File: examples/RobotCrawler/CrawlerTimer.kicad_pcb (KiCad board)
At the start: 2 copper layers, 50 x 62 mm, 38 parts

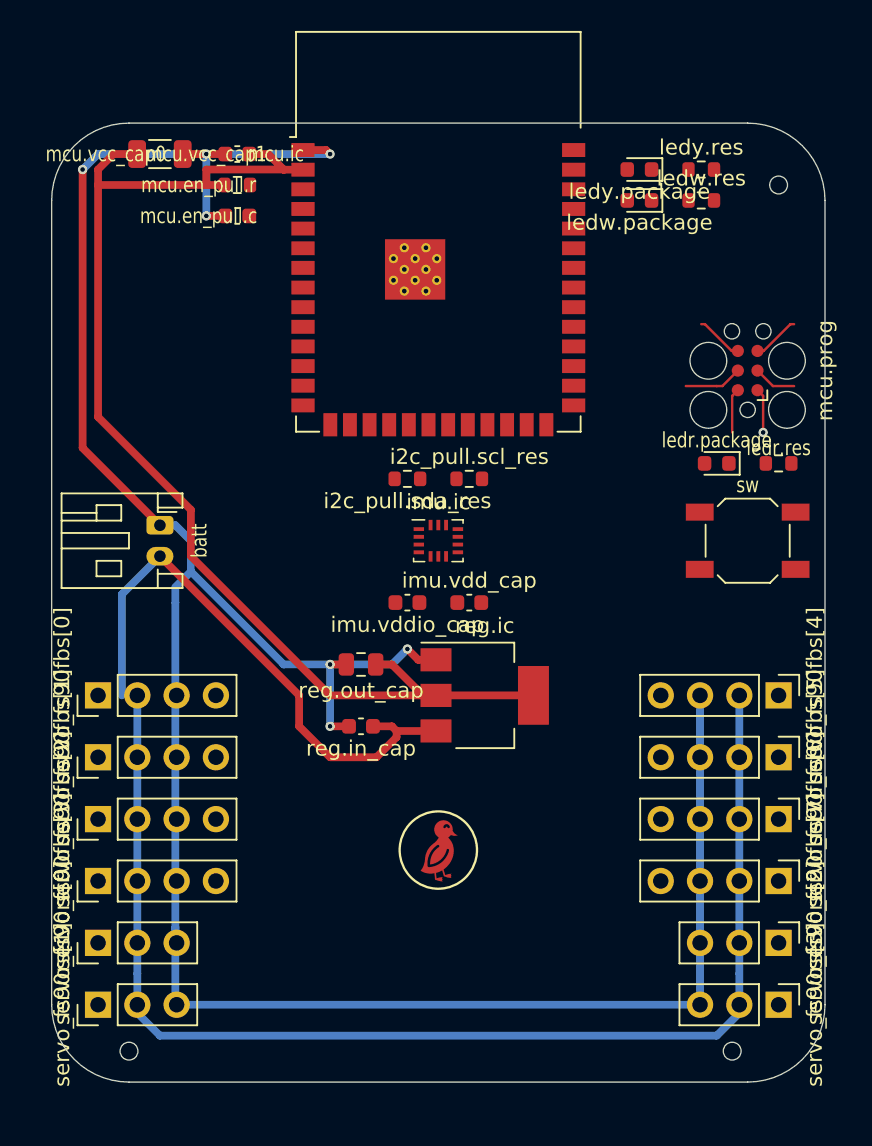
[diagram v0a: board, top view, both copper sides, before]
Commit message: just one copper duck given
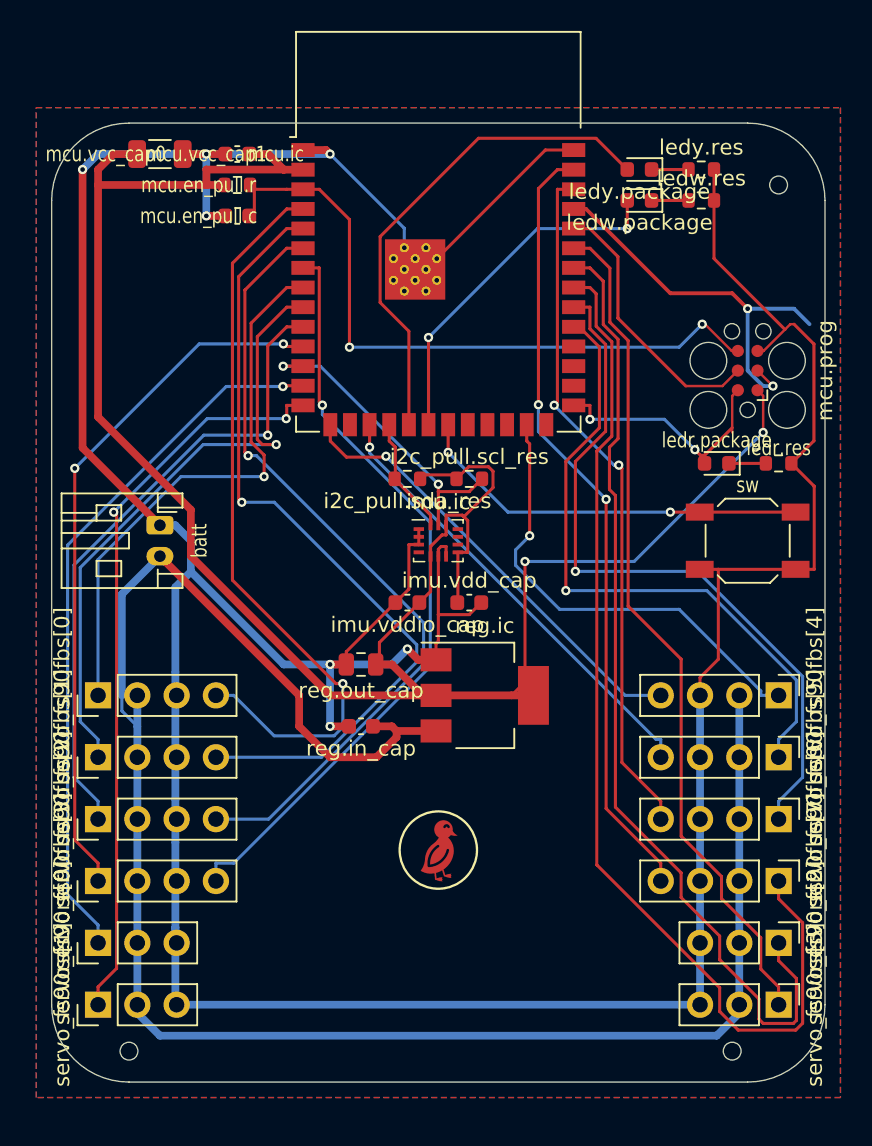
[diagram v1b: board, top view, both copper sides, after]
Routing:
- net batt.gnd: track 167.4 -> 277.2 mm
- net servo_fs90fbs[7].pwm: track 0.00 -> 68.0 mm
- net servo_fs90rs[2].pwm: track 0.00 -> 62.7 mm
- net imu.pwr: track 82.0 -> 138.0 mm, vias 1 -> 2
- net servo_fs90rs[3].pwm: track 0.00 -> 55.0 mm
- net servo_fs90fbs[1].fb: track 0.00 -> 51.9 mm, vias 0 -> 1
- net servo_fs90fbs[2].fb: track 0.00 -> 51.7 mm, vias 0 -> 1
- net servo_fs90fbs[7].fb: track 0.00 -> 50.8 mm, vias 0 -> 2
- net servo_fs90fbs[3].fb: track 0.00 -> 50.1 mm, vias 0 -> 1
- net servo_fs90fbs[0].fb: track 0.00 -> 48.7 mm, vias 0 -> 1
- net servo_fs90rs[1].pwm: track 0.00 -> 48.0 mm, vias 0 -> 2
- net servo_fs90fbs[6].pwm: track 0.00 -> 46.7 mm, vias 0 -> 1
- net servo_fs90rs[0].pwm: track 0.00 -> 46.0 mm, vias 0 -> 1
- net servo_fs90fbs[3].pwm: track 0.00 -> 45.5 mm, vias 0 -> 2
- net servo_fs90fbs[6].fb: track 0.00 -> 44.9 mm, vias 0 -> 2
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- added copper zone on B.Cu, net batt.gnd
- added copper zone on F.Cu, net batt.gnd
